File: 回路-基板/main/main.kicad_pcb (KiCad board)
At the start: 2 copper layers, 63 x 63 mm, 53 parts, among them J1 Conn_01x07_Pin, J2 Conn_01x08_Pin, J3 Conn_01x08_Pin, J4 Conn_01x08_Pin, J5 Conn_01x08_Pin, M1 Jumper_2_Small_Open, M2 Jumper_2_Small_Open, M3 Jumper_2_Small_Open, SW1 SW_Push, SW2 SW_Push, SW3 SW_Push, SW4 SW_Push, SW5 SW_Push, SW8 SW_SPDT, U1 TWE-L-WX, U2 LM1117MP-3.3

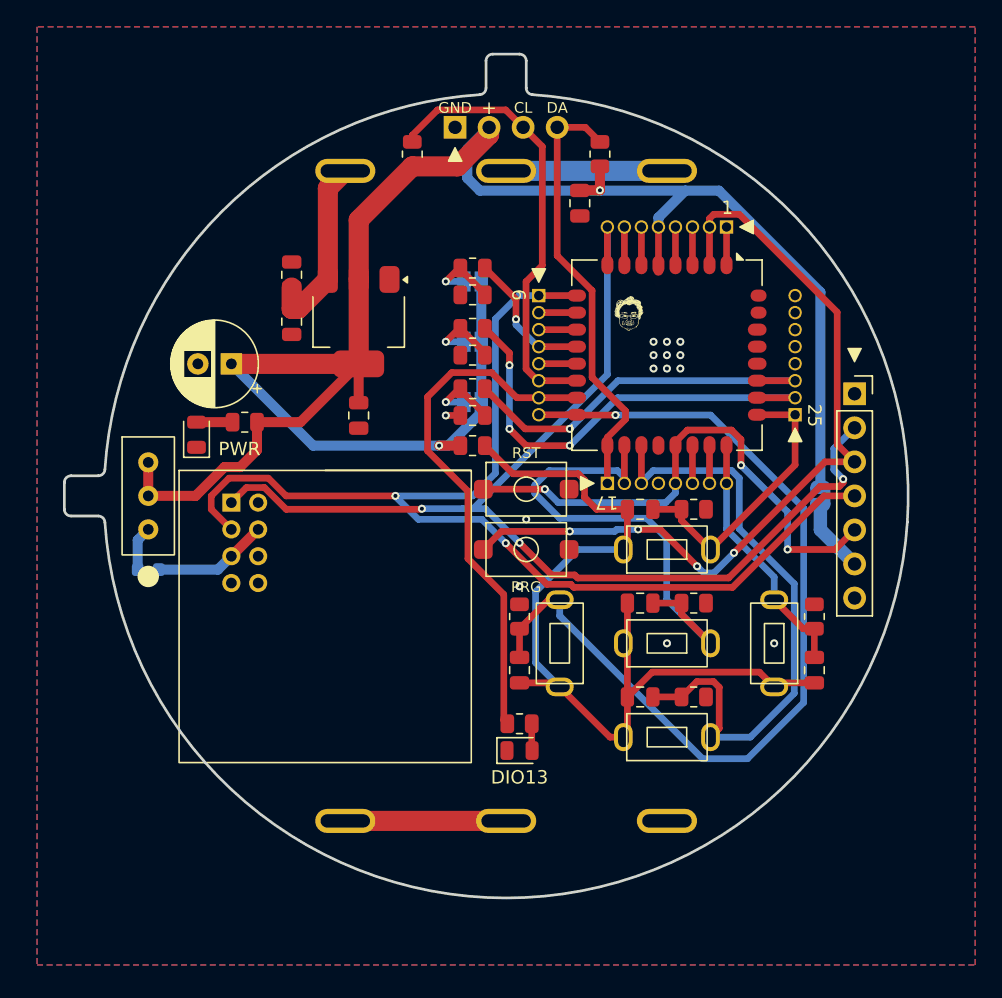
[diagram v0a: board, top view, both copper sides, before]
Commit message: 回路 v3 完成したよ
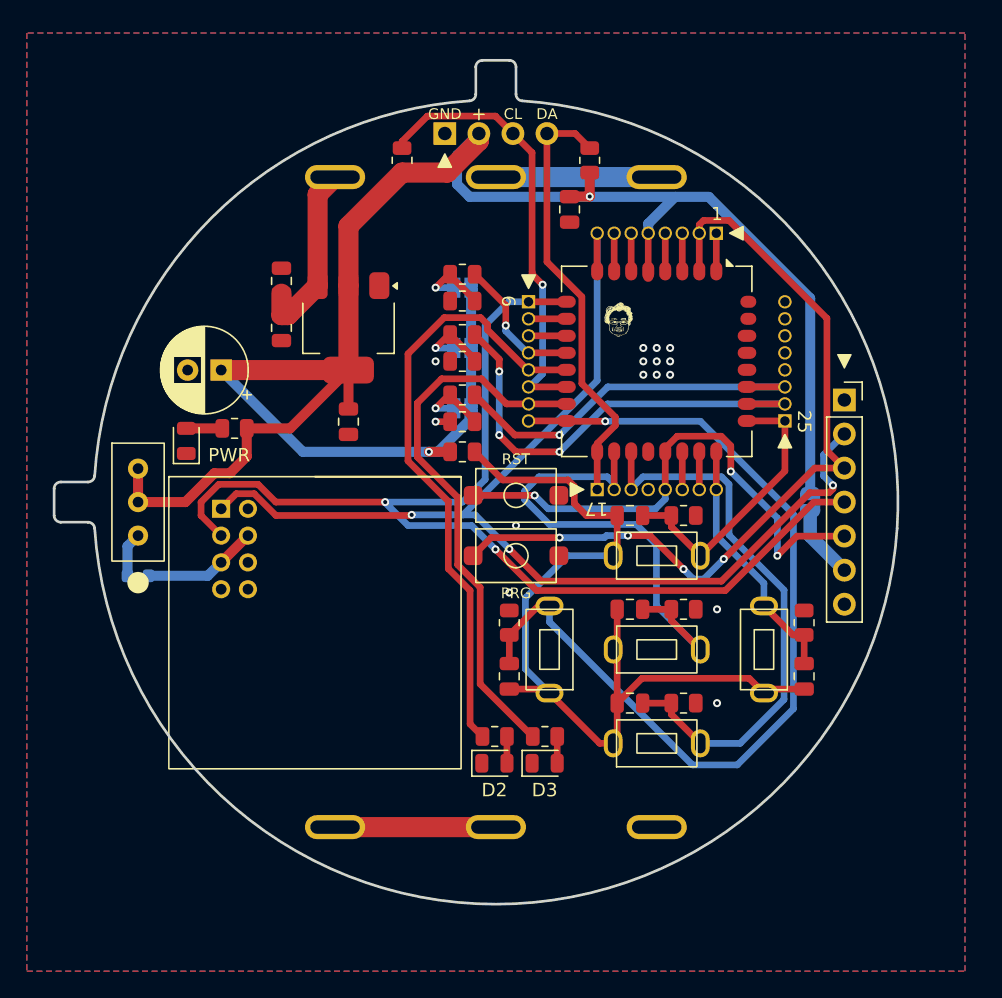
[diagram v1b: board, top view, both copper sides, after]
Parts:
- added D3: LED, LED_SMD:LED_0805_2012Metric, F.Cu at (2.39, 20.0)
- added R17: 330, Resistor_SMD:R_0805_2012Metric, F.Cu at (2.41, 18.0)
- moved D2 2.10 mm to (-1.36, 20.0)
- moved R16 2.08 mm to (-1.34, 18.0)
- moved PWR 0.89 mm to (-24.4, -4.06)
- moved C10 0.89 mm to (4.25, -21.3)
- moved M1 0.89 mm to (-3.75, -15.5)
- moved M2 0.89 mm to (-3.75, -11.0)
- moved M3 0.89 mm to (-3.75, -6.50)
- moved R2 0.89 mm to (-3.75, -14.5)
- moved R3 0.89 mm to (-3.75, -12.0)
- moved R4 0.89 mm to (-3.75, -10.0)
- moved R5 0.89 mm to (-3.75, -7.50)
- moved R6 0.89 mm to (-3.75, -5.50)
- moved SW3 0.89 mm to (2.75, 11.5)
- moved J2 0.89 mm to (15.2, -19.6)
- moved J4 0.89 mm to (6.30, -0.44)
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- renumbered DIO13 to D2
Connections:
- R16 pad 1: 15 -> 13
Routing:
- net 13: track 2.83 -> 45.6 mm
- net 19: track 45.8 -> 42.2 mm
- net Net-(D3-A): track 0.00 -> 2.00 mm
- net 15: track 39.5 -> 41.1 mm
- net 14: track 33.4 -> 33.3 mm, vias 0 -> 1
- net GND: track 1.12 -> 1.09 mm, vias 14 -> 15
